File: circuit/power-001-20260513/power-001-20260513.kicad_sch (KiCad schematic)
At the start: 34 parts, among them J1 VIN, Q1 NMOS, Q2 PMOS, SW1 SW_SPST, U1 PIC12F683-xSN

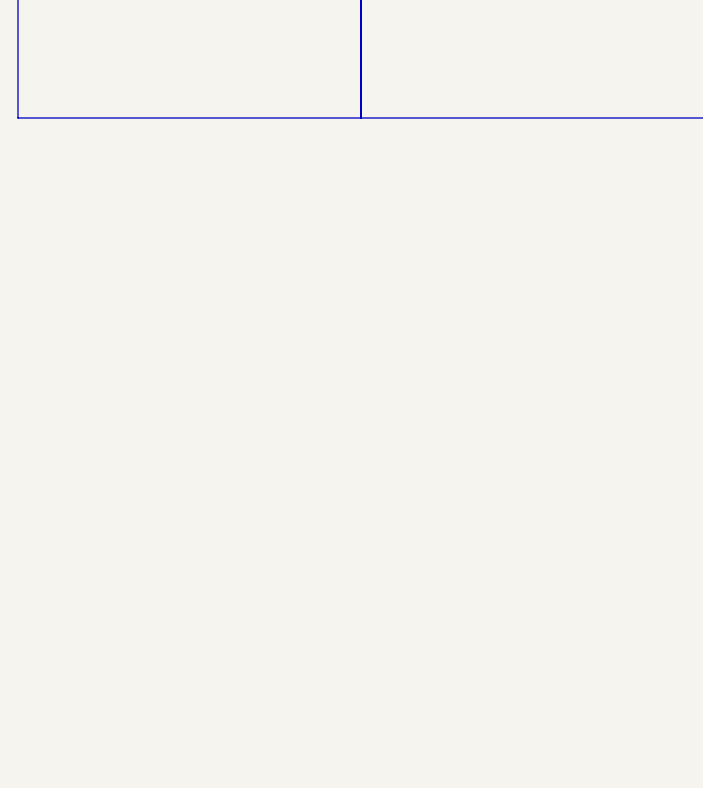
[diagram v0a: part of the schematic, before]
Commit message: Update メイン基板の発注ファイルを更新
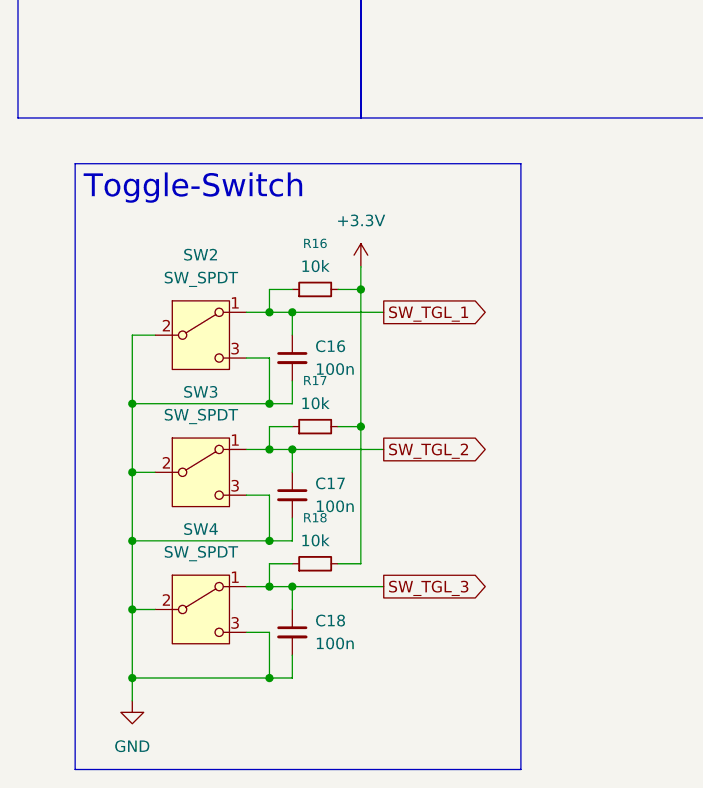
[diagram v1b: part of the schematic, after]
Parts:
- added C16, C17, C18: 100n, Capacitor_SMD:C_0805_2012Metric, symbol Device:C_Small
- added R16, R17, R18: 10k, Resistor_SMD:R_0805_2012Metric, symbol Device:R_Small
- added SW2, SW3, SW4: SW_SPDT, symbol Switch:SW_SPDT
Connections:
- net +3.3V: now also R16.2, R17.2, R18.2
- net GND: now also C16.2, C17.2, C18.2, SW2.2 (B), SW2.3 (C), SW3.2 (B), SW3.3 (C), SW4.2 (B), SW4.3 (C)
- new net SW_TGL_1: C16.1, R16.1, SW2.1 (A)
- new net SW_TGL_2: C17.1, R17.1, SW3.1 (A)
- new net SW_TGL_3: C18.1, R18.1, SW4.1 (A)

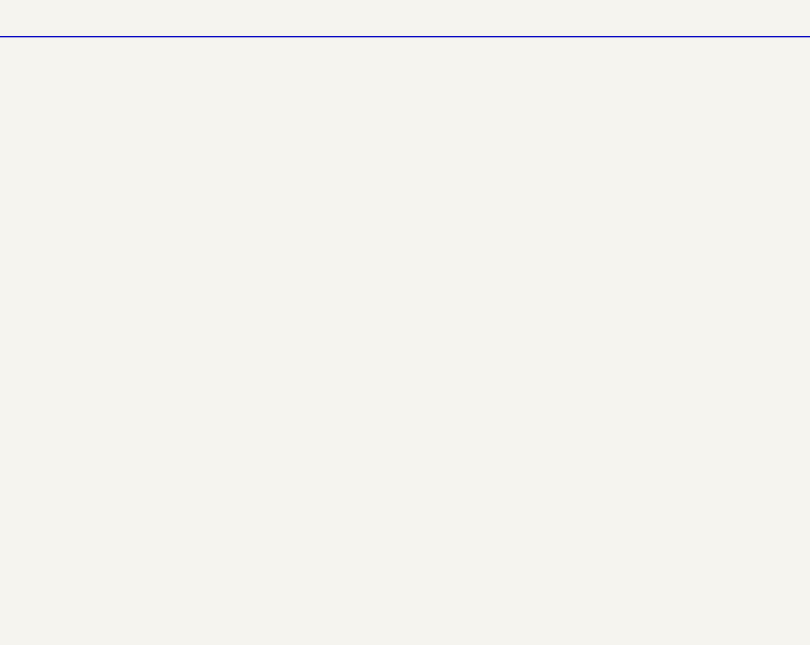
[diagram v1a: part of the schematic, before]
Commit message: Update サブ基板の回路図が完成した
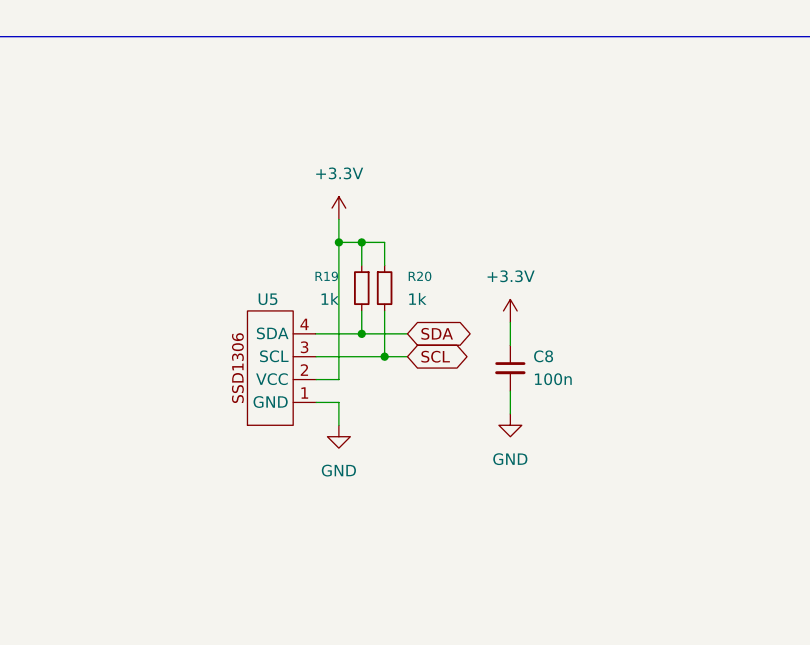
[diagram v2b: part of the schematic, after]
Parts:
- added C8: 100n, Capacitor_SMD:C_0805_2012Metric, symbol Device:C_Small
- added R19, R20: 1k, Resistor_SMD:R_0805_2012Metric, symbol Device:R_Small
- added U5: (no value), symbol @Thrive_symbol_sub:SSD1306
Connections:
- net +3.3V: now also C8.1, R19.1, R20.1, U5.2 (VCC)
- net GND: now also C8.2, U5.1 (GND)
- new net SCL: R20.2, U5.3 (SCL)
- new net SDA: R19.2, U5.4 (SDA)
